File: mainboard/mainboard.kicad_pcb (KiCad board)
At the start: 2 copper layers, 110 x 90 mm, 81 parts, among them K1 G6S-2F-5DC, X1 POWER, X10 BUTTONS, X2 IO, X3 INPUT, X4 FRONT INPUT, X5 MAIN OUTPUT, X6 PHONES OUTPUT, X7 UART, X8 DISPLAY, X9 ENCODER

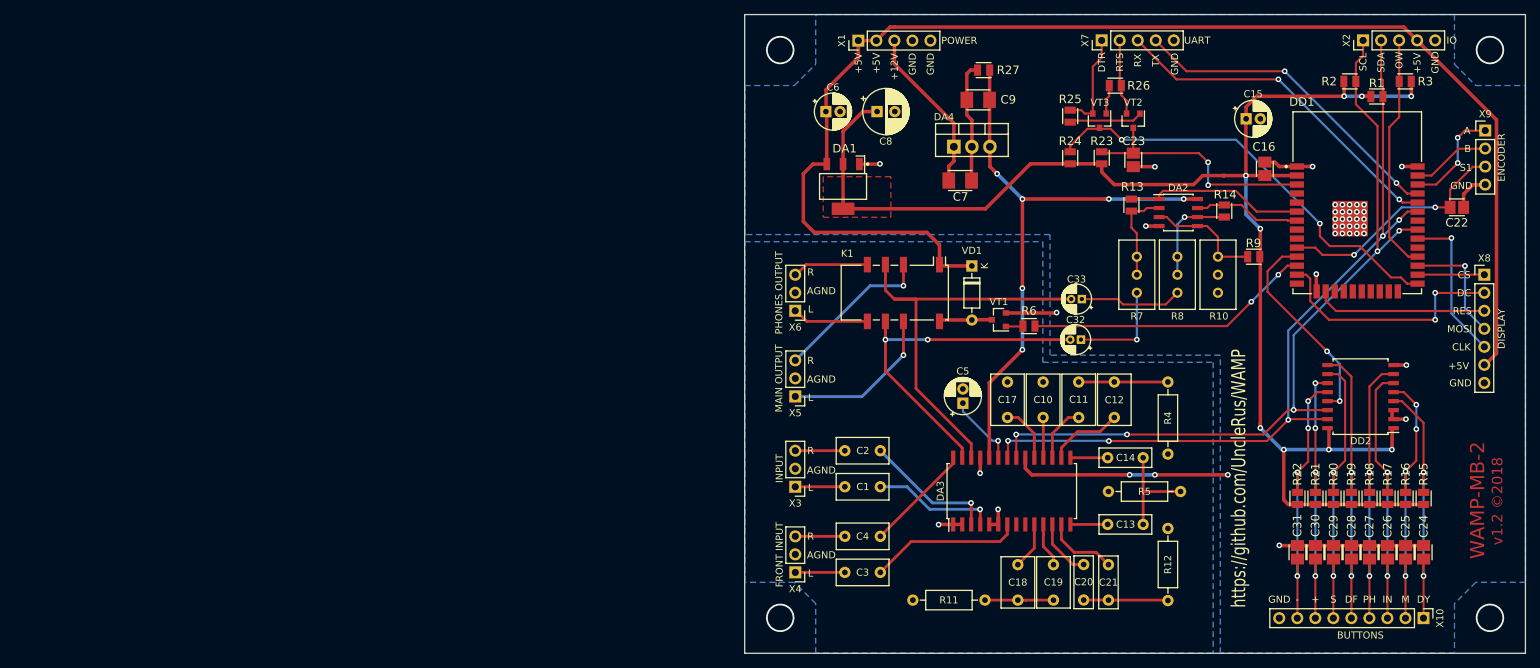
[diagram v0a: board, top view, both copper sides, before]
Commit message: v1.3
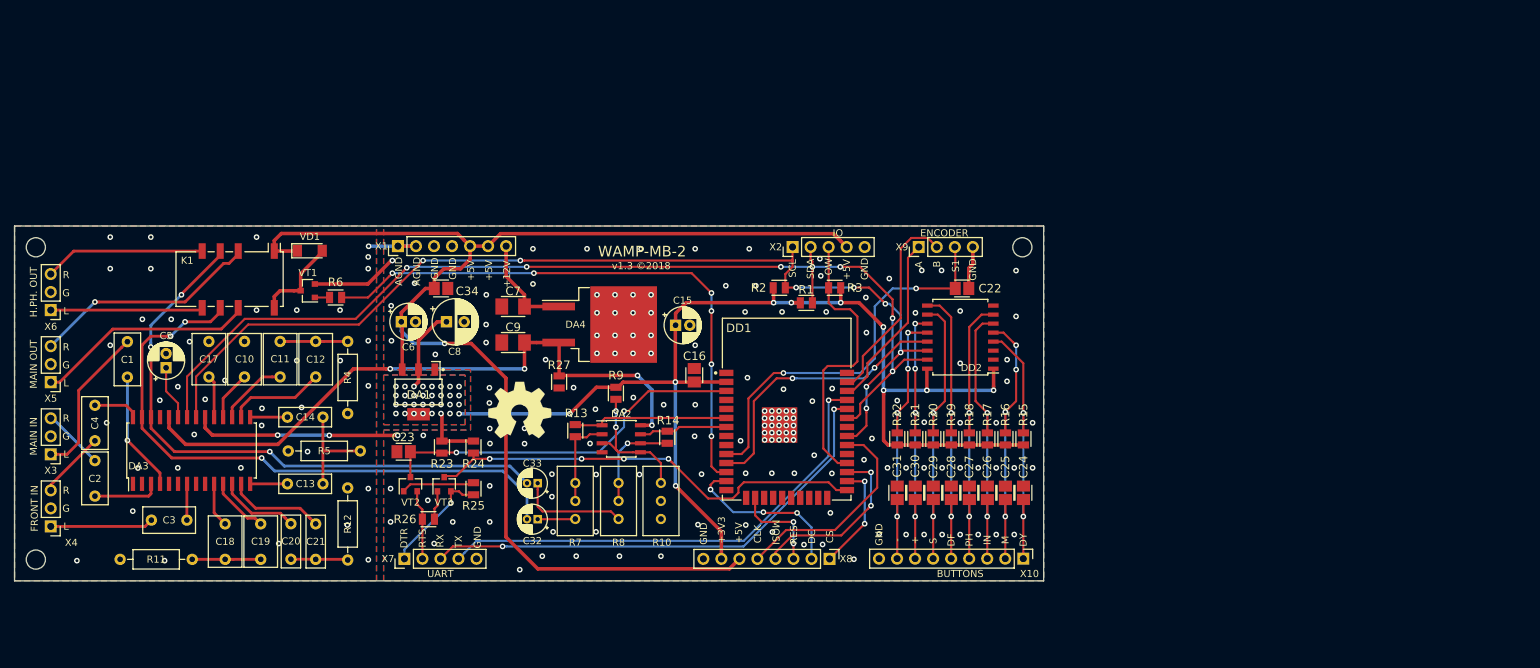
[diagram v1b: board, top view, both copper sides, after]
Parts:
- added C34: 100n, WAMP:CAPC2013X140N, F.Cu at (44.2, 74.4)
- added REF**: OSHW-Symbol_8.9x8mm_SilkScreen, Symbol:OSHW-Symbol_8.9x8mm_SilkScreen, F.Cu at (55.3, 91.5)
- added REF**: MountingHole_2.7mm_M2.5_DIN965, MountingHole:MountingHole_2.7mm_M2.5_DIN965, F.Cu at (126.1, 68.6)
- added REF**: MountingHole_2.7mm_M2.5_DIN965, MountingHole:MountingHole_2.7mm_M2.5_DIN965, F.Cu at (-12.9, 112.6)
- added REF**: MountingHole_2.7mm_M2.5_DIN965, MountingHole:MountingHole_2.7mm_M2.5_DIN965, F.Cu at (-12.9, 68.6)
- DA4: footprint Package_TO_SOT_THT:TO-220-3_Vertical -> Package_TO_SOT_SMD:TO-263-2
- VD1: footprint Diode_THT:D_DO-35_SOD27_P7.62mm_Horizontal -> Diode_SMD:D_MiniMELF
- X1: footprint Connector_PinHeader_2.54mm:PinHeader_1x05_P2.54mm_Vertical -> Connector_PinHeader_2.54mm:PinHeader_1x07_P2.54mm_Vertical
- X8: footprint Connector_PinHeader_2.54mm:PinHeader_1x07_P2.54mm_Vertical -> Connector_PinHeader_2.54mm:PinHeader_1x08_P2.54mm_Vertical
- moved X7 122.4 mm to (39.1, 112.5)
- moved R12 115.7 mm to (31.1, 112.7)
- moved R4 115.7 mm to (31.1, 92.0)
- moved R5 115.7 mm to (22.7, 97.3)
- moved C13 115.7 mm to (27.6, 101.9)
- moved C14 115.7 mm to (27.6, 92.5)
- moved DA3 115.7 mm to (9.09, 97.2)
- moved R26 114.4 mm to (42.5, 106.9), turned to 270 degrees
- moved VT2 114.0 mm to (39.9, 102.0), turned to 90 degrees
- moved C11 112.7 mm to (21.6, 81.9)
- moved C12 112.7 mm to (26.6, 81.9)
- moved C17 112.7 mm to (11.5, 81.9)
- moved C10 112.7 mm to (16.5, 81.9)
- moved C5 112.4 mm to (5.50, 85.6)
- moved C18 111.8 mm to (13.8, 112.6)
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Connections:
- C7 pad 1: Net-(C7-Pad1) -> /12V
- DA4 pad 1: Net-(C7-Pad1) -> /12V
- X1 pad 1: +5V -> AGND
- X1 pad 2: +5V -> AGND
- X1 pad 3: Net-(C7-Pad1) -> GND
- X1 pad 5: GND -> +5V
- X8 pad 7: GND -> +3V3
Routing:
- net GND: track 105.2 -> 47.5 mm, vias 38 -> 154
- net /PH_SW: track 40.4 -> 81.6 mm, vias 2 -> 6
- net /LOUT: track 49.6 -> 87.0 mm, vias 2 -> 3
- net /SDA: track 114.3 -> 147.1 mm, vias 5 -> 7
- net /SCL: track 114.4 -> 145.4 mm, vias 5 -> 8
- net /ROUT: track 58.7 -> 85.2 mm, vias 0 -> 3
- net Net-(C7-Pad1): track 23.5 -> 0.00 mm
- net +3V3: track 214.7 -> 191.6 mm, vias 9 -> 42
- net /TXD: track 45.8 -> 68.6 mm, vias 2 -> 1
- net /RE_BTN: track 33.5 -> 56.1 mm
- net /RXD: track 48.9 -> 69.9 mm
- net /EN: track 34.7 -> 52.8 mm
- net /RE_B: track 11.0 -> 28.7 mm
- net Net-(C3-Pad2): track 21.5 -> 5.12 mm
- net Net-(C1-Pad1): track 6.98 -> 21.7 mm
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- added copper zone on B.Cu, net +3V3
- added copper zone on F.Cu, net AGND
- added copper zone on F.Cu, net GND
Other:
- board size 110 x 90 mm -> 145 x 50 mm
- board text added: "+3V3"
- board text added: "FRONT IN"
- board text added: "G"
- board text added: "H.PH. OUT"
- board text added: "MAIN IN"
- board text added: "MAIN OUT"
- board text added: "v1.3 ©2018"
- board text removed: "https://github.com/UncleRus/WAMP"
- board text removed: "v1.2 ©2018"
